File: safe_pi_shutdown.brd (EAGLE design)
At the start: 65 x 56 mm, 31 parts, among them U1 LTC2952CF

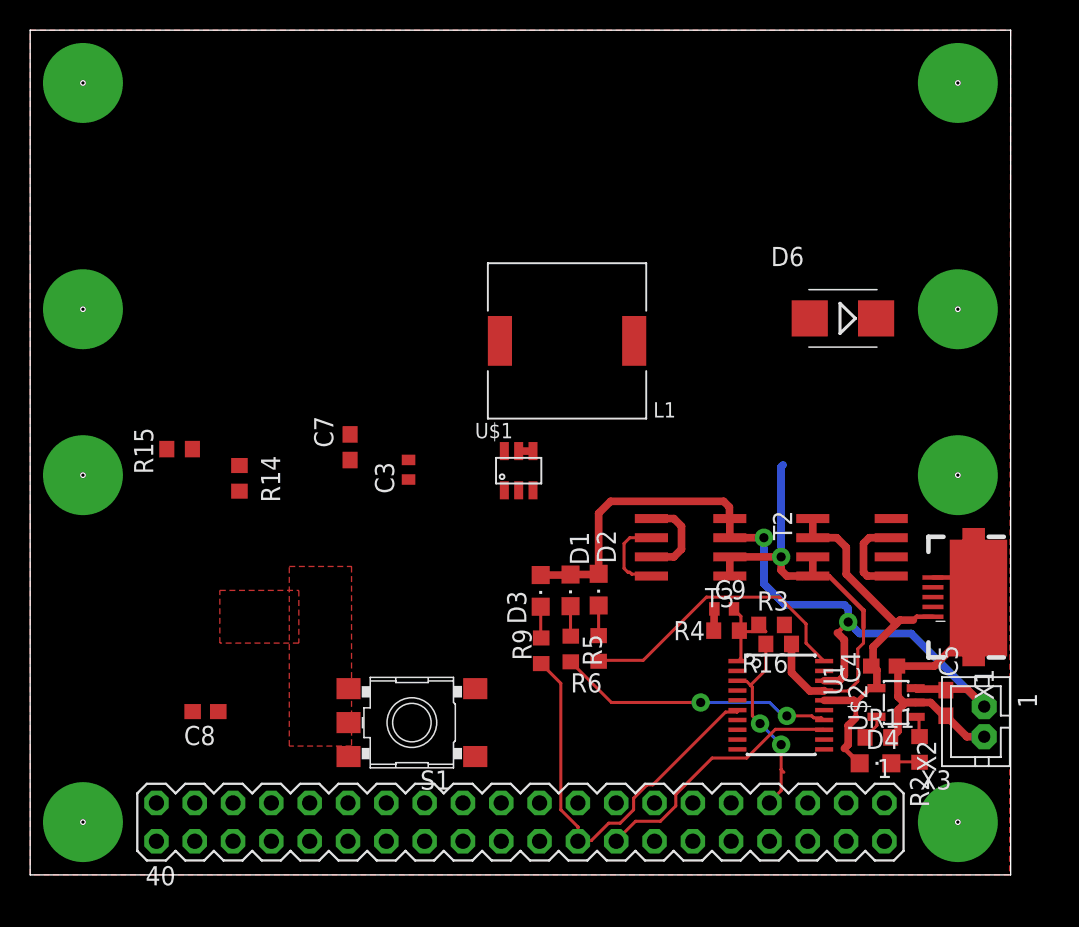
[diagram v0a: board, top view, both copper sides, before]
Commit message: prawie pierwsza wersja
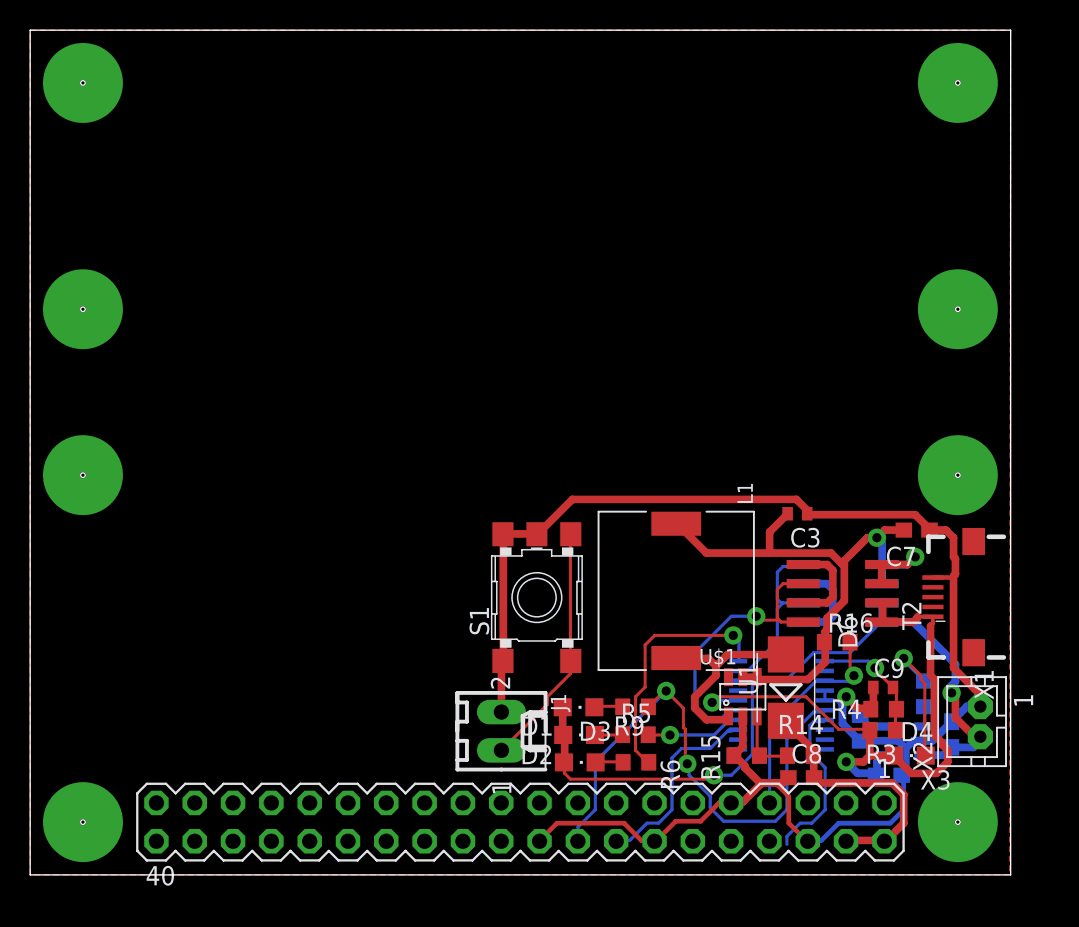
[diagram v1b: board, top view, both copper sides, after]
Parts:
- added J1: 22-27-2021-02, con-molex:6410-02
- moved R15 42.7 mm to (47.5, 7.91)
- moved R14 41.5 mm to (51.1, 7.91), turned to 180 degrees
- moved C8 39.7 mm to (51.1, 6.45), turned to 180 degrees
- moved C7 38.0 mm to (58.8, 22.9), turned to 0 degrees
- moved C3 25.9 mm to (50.9, 23.9), turned to 180 degrees
- moved D6 24.8 mm to (50.1, 12.4), turned to 90 degrees
- moved U$1 21.1 mm to (47.2, 11.8)
- moved L1 18.1 mm to (42.8, 18.8), turned to 0 degrees
- moved C9 11.8 mm to (56.5, 12.4)
- moved S1 11.7 mm to (33.6, 18.4), turned to 90 degrees
- moved R4 11.6 mm to (56.6, 11.0)
- moved D2 11.5 mm to (36.4, 7.46), turned to 270 degrees
- moved T3 10.5 mm to (53.9, 18.7), flipped to the bottom, turned to 90 degrees
- moved R3 10.2 mm to (56.5, 9.59), turned to 180 degrees
- moved D1 9.60 mm to (36.4, 9.28), turned to 270 degrees
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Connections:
- removed net N$7: S1.3, U1.7
- new net N$5: J1.1, S1.3, S1.4, U1.7
- net GND: now also J1.2, X2.1; no longer X2.2
- net V1: now also X2.2; no longer X2.1
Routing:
- net GND: track 23.7 -> 116.8 mm, vias 0 -> 1
- net N$5: track 0.00 -> 27.2 mm
- net N$3: track 0.00 -> 19.2 mm, vias 0 -> 1
- net N$4: track 0.00 -> 17.2 mm
- net V2: track 26.7 -> 41.8 mm, vias 0 -> 2
- net N$13: track 0.00 -> 13.8 mm
- net N$17: track 18.4 -> 6.38 mm, vias 2 -> 1
- net VCC: track 32.6 -> 43.2 mm, vias 1 -> 2
- net N$18: track 27.4 -> 36.7 mm, vias 0 -> 2
- net N$6: track 1.93 -> 9.23 mm, vias 0 -> 1
- net N$2: track 5.65 -> 11.7 mm
- net N$21: track 0.00 -> 4.55 mm
- net N$10: track 17.3 -> 13.8 mm
- net N$19: track 19.2 -> 16.4 mm, vias 0 -> 1
- net N$8: track 6.17 -> 8.25 mm, vias 0 -> 1
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- removed copper zone on layer 1, net V2
